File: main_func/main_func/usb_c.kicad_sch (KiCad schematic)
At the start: 6 parts, among them J1 USB_C_Receptacle_USB2.0, J2 Conn_01x04_Male

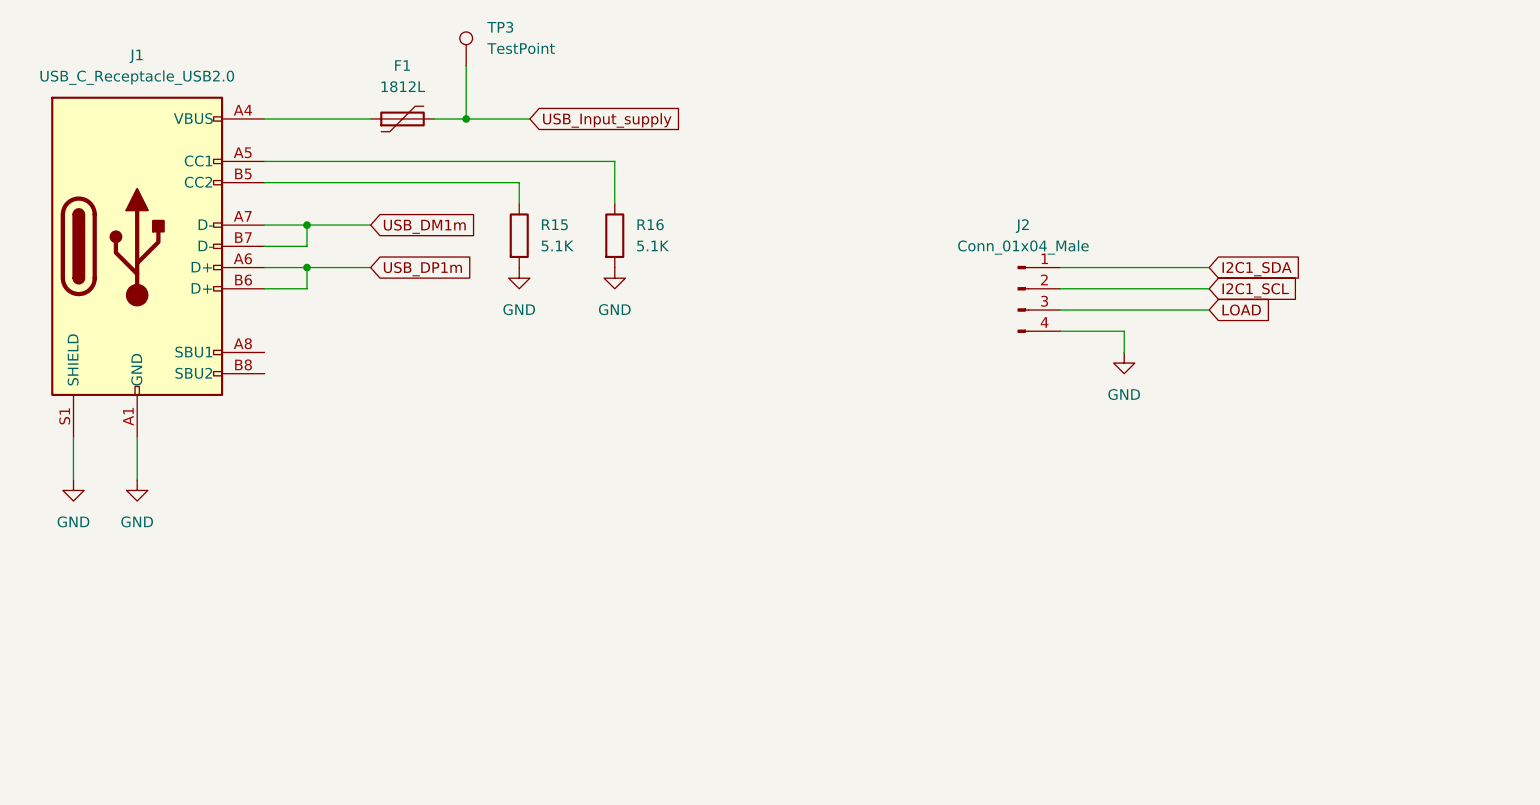
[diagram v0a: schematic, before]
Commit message: pcb design fixing
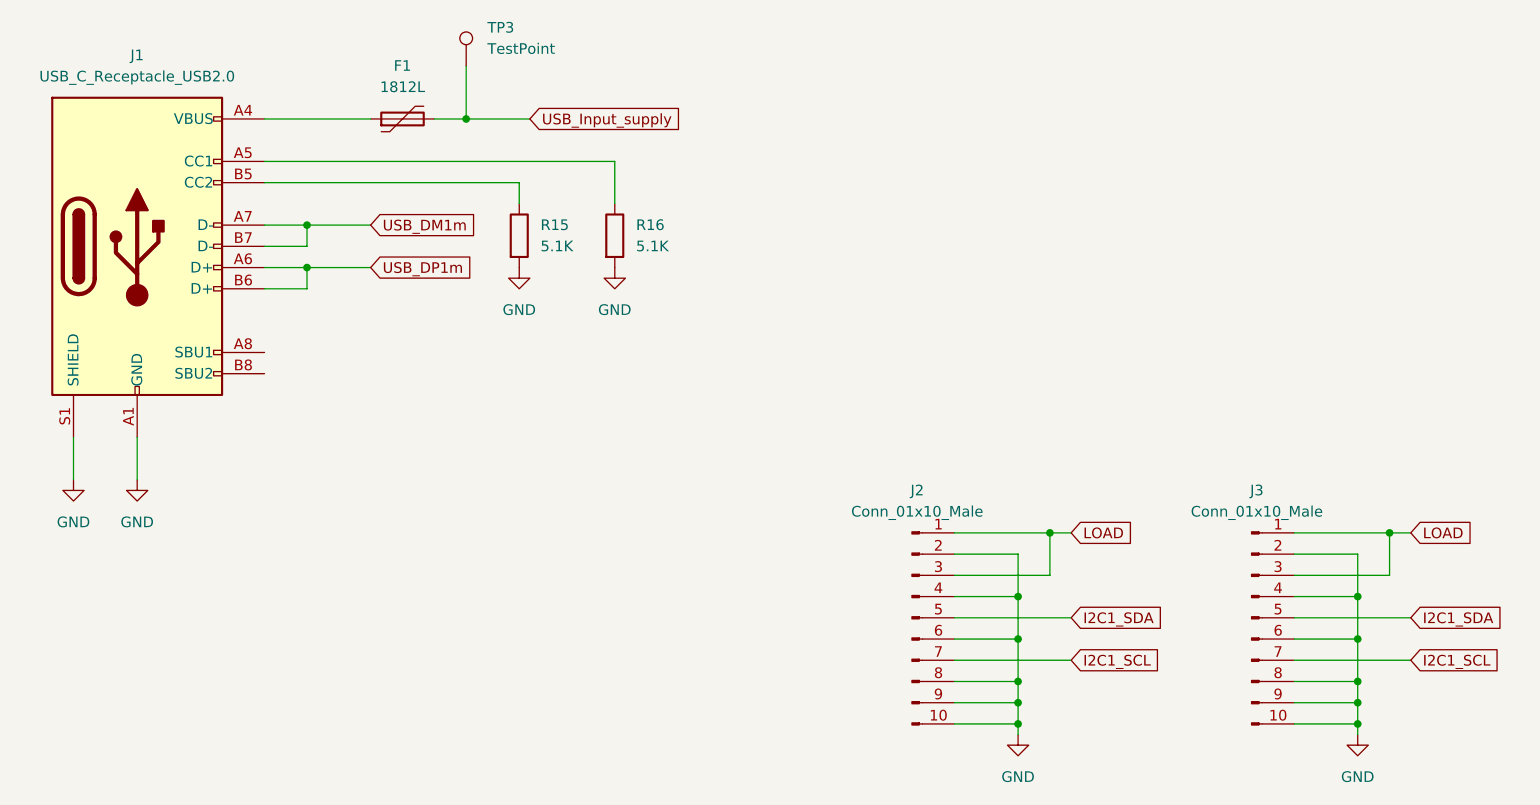
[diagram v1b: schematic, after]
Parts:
- removed J2: Conn_01x04_Male, Connector_PinHeader_2.54mm:PinHeader_1x04_P2.54mm_Horizontal, symbol Connector:Conn_01x04_Male
- added J2, J3: Conn_01x10_Male, Connector_IDC:IDC-Header_2x05_P2.54mm_Horizontal, symbol Connector:Conn_01x10_Male
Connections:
- net GND: now also J2.10 (Pin_10), J2.2 (Pin_2), J2.4 (Pin_4), J2.6 (Pin_6), J2.8 (Pin_8), J2.9 (Pin_9), J3.10 (Pin_10), J3.2 (Pin_2), J3.4 (Pin_4), J3.6 (Pin_6), J3.8 (Pin_8), J3.9 (Pin_9)
- net I2C1_SCL: now also J2.7 (Pin_7), J3.7 (Pin_7)
- net I2C1_SDA: now also J2.5 (Pin_5), J3.5 (Pin_5)
- net LOAD: now also J2.1 (Pin_1), J2.3 (Pin_3), J3.1 (Pin_1), J3.3 (Pin_3)
